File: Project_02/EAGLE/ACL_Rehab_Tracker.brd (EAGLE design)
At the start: 100 x 80 mm, 18 parts, among them U1 POCKETBEAGLE, U2 MPU-6050-A

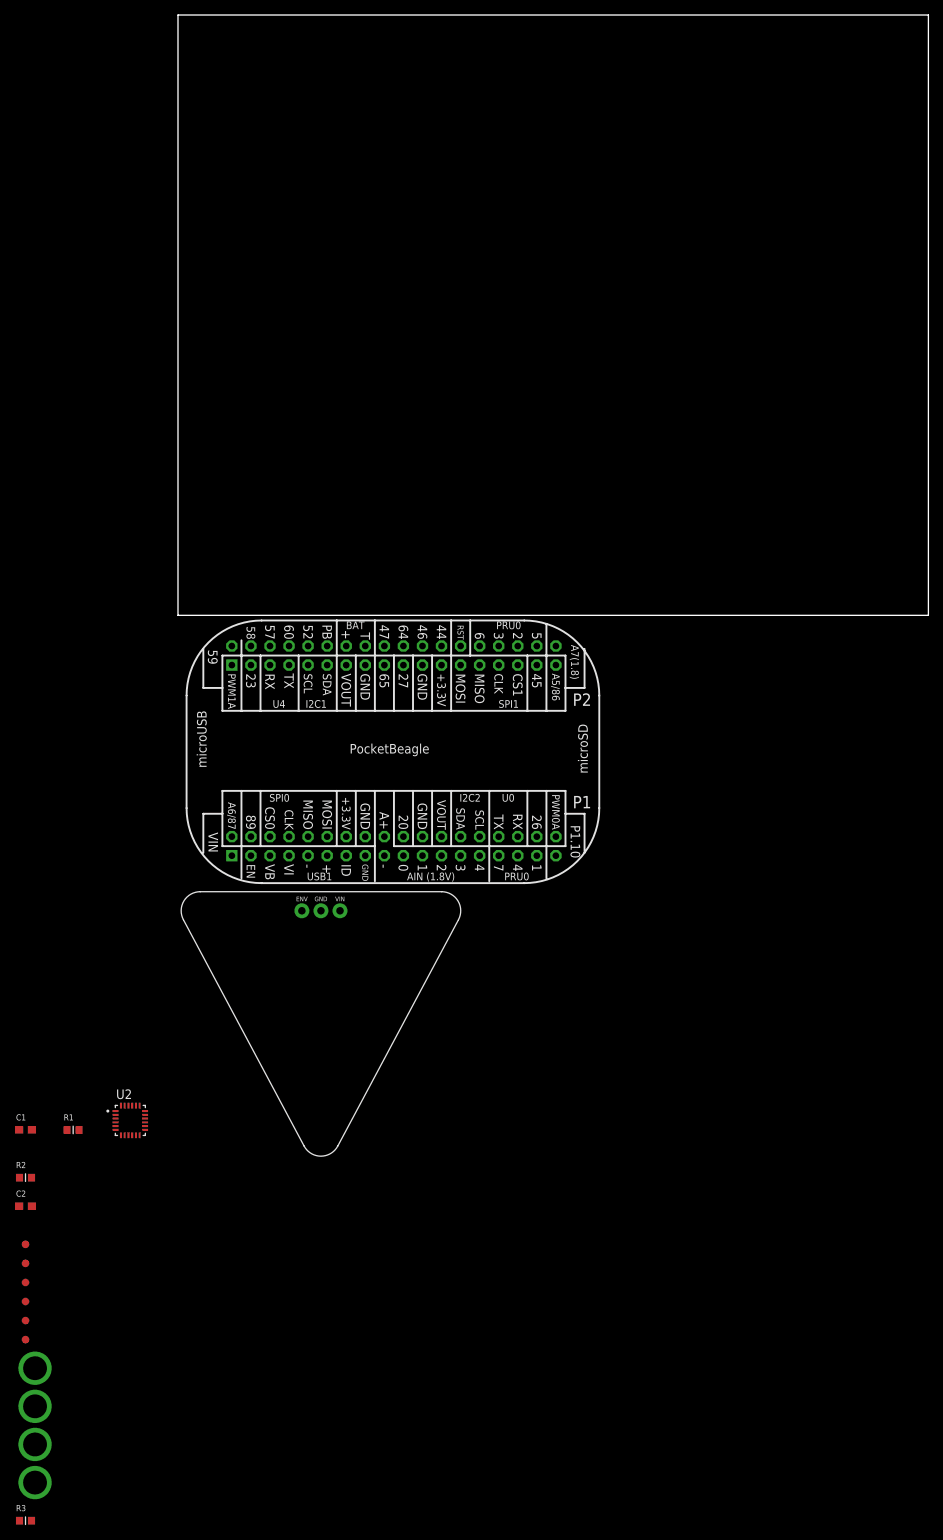
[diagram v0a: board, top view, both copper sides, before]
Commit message: Final Project_02
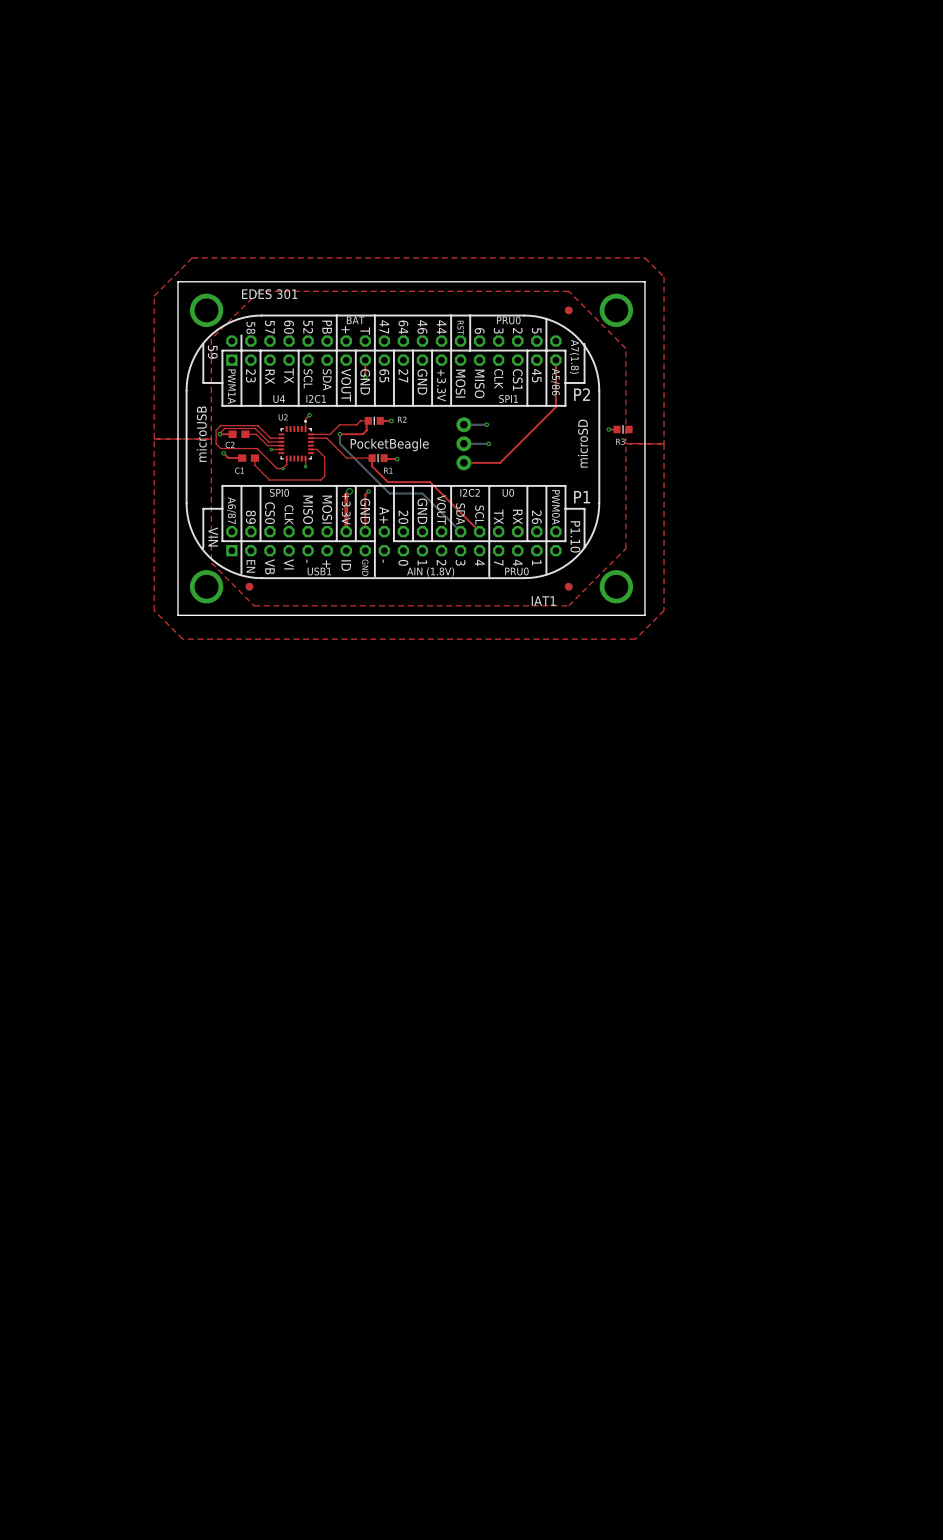
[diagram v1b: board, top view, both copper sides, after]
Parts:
- moved MGT4 174.4 mm to (58.4, 40.6)
- moved R3 165.8 mm to (59.3, 24.8)
- moved FUD4 150.6 mm to (52.1, 40.6), flipped to the bottom
- moved FUD3 148.4 mm to (52.1, 40.6)
- moved MGT1 142.8 mm to (3.81, 40.6)
- moved MGT3 138.1 mm to (58.4, 3.81)
- moved FUD5 121.7 mm to (52.1, 3.81), flipped to the bottom
- moved FUD2 115.6 mm to (52.1, 3.81)
- moved MGT2 111.6 mm to (3.81, 3.81)
- moved R2 111.0 mm to (26.2, 25.9)
- moved C2 106.7 mm to (8.13, 24.1), turned to 180 degrees
- moved FUD6 104.7 mm to (9.53, 3.81), flipped to the bottom
- moved R1 98.3 mm to (26.7, 21.0), turned to 180 degrees
- moved C1 94.3 mm to (9.40, 21.0), turned to 180 degrees
- moved U2 92.8 mm to (15.7, 22.9), turned to 270 degrees
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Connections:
- removed net VOUT: U1.P1_24, U1.P2_13
- new net N$3: U1.P2_13
- new net N$4: U1.P1_24
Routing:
- net I2C_SDA: track 0.00 -> 35.6 mm, vias 0 -> 1
- net VDD_3P3V: track 0.00 -> 35.1 mm, vias 0 -> 5
- net GND: track 0.00 -> 30.4 mm, vias 0 -> 9
- net I2C_SCL: track 0.00 -> 28.3 mm
- net MYOWARE: track 0.00 -> 21.6 mm
- net N$1: track 0.00 -> 16.1 mm
- net N$2: track 0.00 -> 5.43 mm
- added copper zone on layer 1, net CGND
- added copper zone on layer 2, net GND
- added copper zone on layer 15, net VDD_3P3V
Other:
- board size 100 x 80 mm -> 62.2 x 44.5 mm
- board text added: "EDES 301"
- board text added: "IAT1"
